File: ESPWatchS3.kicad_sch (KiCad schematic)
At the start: 128 parts

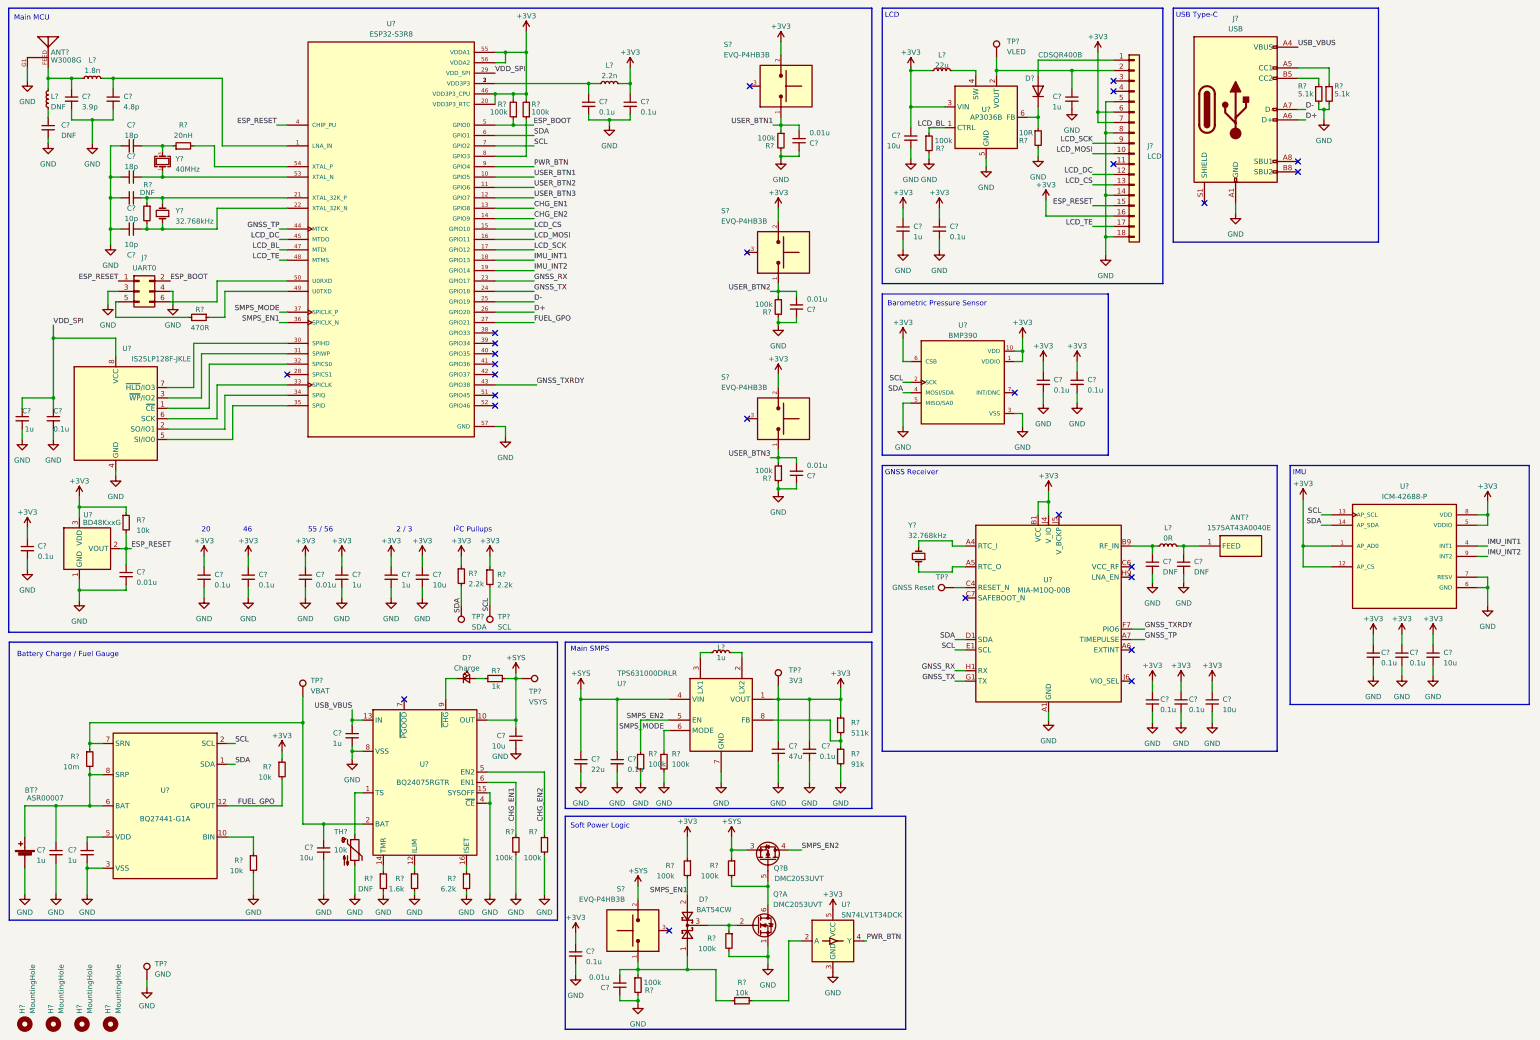
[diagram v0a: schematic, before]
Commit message: Re-annotated schematic
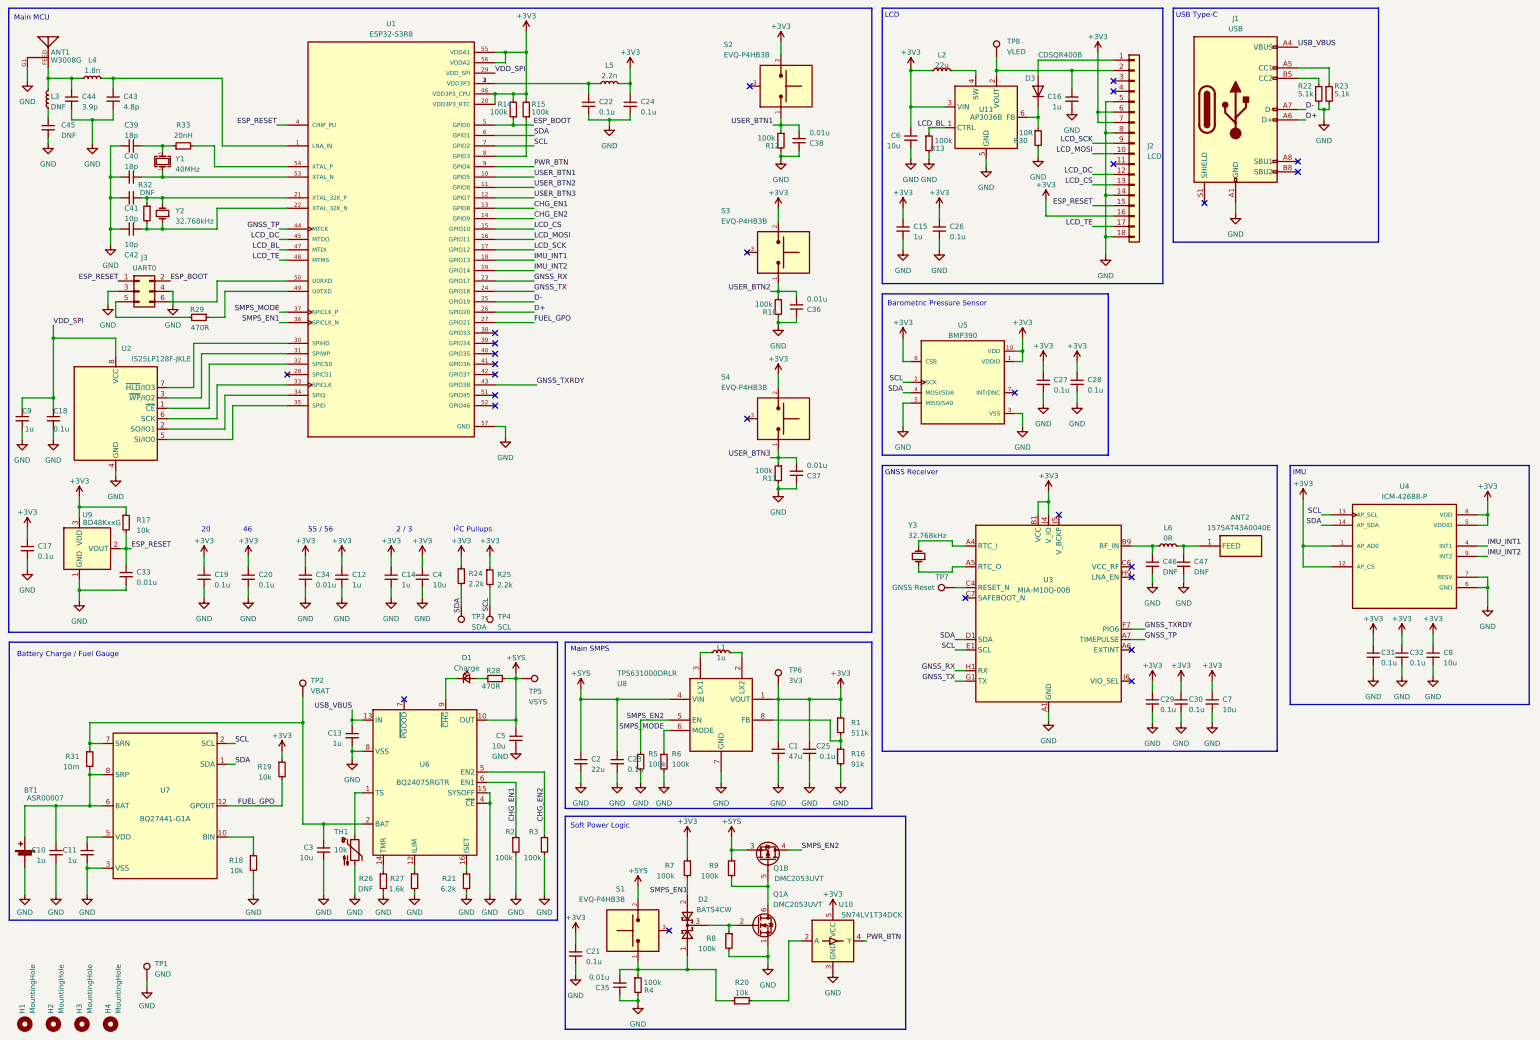
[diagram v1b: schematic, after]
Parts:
- R28: renamed from R?; value 1k -> 470R
- gave numbers to parts that had none: 126

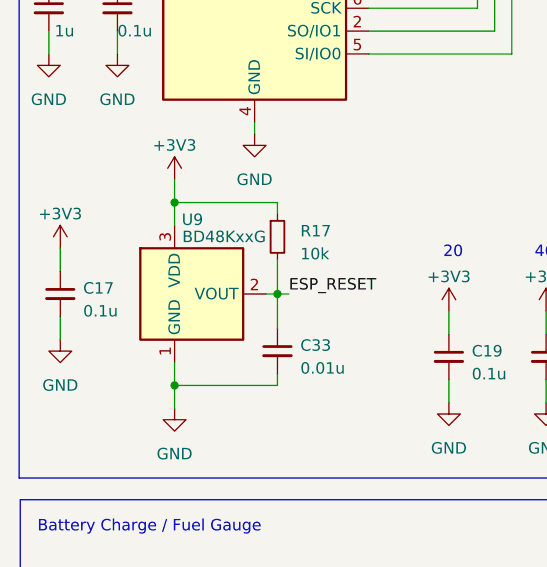
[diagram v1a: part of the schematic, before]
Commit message: Finished Footprint Assignment
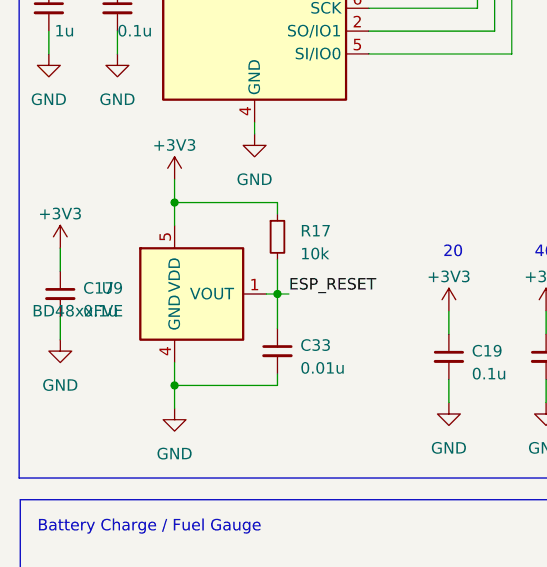
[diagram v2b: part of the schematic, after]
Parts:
- removed U9: BD48KxxG, Package_TO_SOT_SMD:SOT-23, symbol Power_Management:BD48KxxG
- added U9: BD48xxFVE, Package_TO_SOT_SMD:VSOF5, symbol Power_Management:BD48xxFVE
- J2: footprint (none) -> WatchParts:CS050Z18GA0
- L2: footprint (none) -> Inductor_SMD:L_1210_3225Metric
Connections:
- net +3V3: now also U9.5 (VDD)
- net EP: now also U9.2 (GND), U9.4 (GND)
- net ESP_RESET: now also U9.1 (VOUT)
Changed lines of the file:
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@@
       (effects (font (size 1.27 1.27)) (justify left))
     )
-    (property "Footprint" "" (at 288.925 46.99 0)
+    (property "Footprint" "WatchParts:CS050Z18GA0" (at 288.925 46.99 0)
       (effects (font (size 1.27 1.27)) hide)
     )
@@
       (effects (font (size 1.27 1.27)))
     )
-    (property "Footprint" "" (at 241.935 29.21 0)
+    (property "Footprint" "Inductor_SMD:L_1210_3225Metric" (at 241.935 29.21 0)
       (effects (font (size 1.27 1.27)) hide)
     )
@@
     )
   )
-  (symbol (lib_id "Power_Management:BD48KxxG") (at 31.115 146.05 0) (unit 1)
-    (in_bom yes) (on_board yes) (dnp no)
-    (property "Reference" "U9" (at 34.29 137.795 0)
-      (effects (font (size 1.27 1.27)) (justify right))
-    )
-    (property "Value" "BD48KxxG" (at 41.275 139.7 0)
-      (effects (font (size 1.27 1.27)) (justify right))
-    )
-    (property "Footprint" "Package_TO_SOT_SMD:SOT-23" (at 31.115 158.75 0)
-      (effects (font (size 1.27 1.27)) hide)
-    )
-    (property "Datasheet" "https://www.rohm.de/datasheet/BD4830FVE/bd48xxg-e" (at 31.115 161.29 0)
-      (effects (font (size 1.27 1.27)) hide)
-    )
-    (pin "1")
-    (pin "2")
-    (pin "3")
-    (instances
-      (project "ESPWatchS3"
-        (path "/bf5b2c41-bb33-4360-ba29-22d569e03292"
-          (reference "U9") (unit 1)
-        )
-      )
-    )
-  )
   (symbol (lib_id "Device:R_Small") (at 217.17 196.85 0) (unit 1)
     (in_bom yes) (on_board yes) (dnp no) (fields_autoplaced)
@@
         )
       )
+    )
+  )
+  (symbol (lib_id "Power_Management:BD48xxFVE") (at 31.115 146.05 0) (unit 1)
+    (in_bom yes) (on_board yes) (dnp no) (fields_autoplaced)
+    (property "Reference" "U9" (at 25.4 145.415 0)
+      (effects (font (size 1.27 1.27)) (justify right))
+    )
+    (property "Value" "BD48xxFVE" (at 25.4 147.955 0)
+      (effects (font (size 1.27 1.27)) (justify right))
+    )
+    (property "Footprint" "Package_TO_SOT_SMD:VSOF5" (at 31.115 158.75 0)
+      (effects (font (size 1.27 1.27)) hide)
+    )
+    (property "Datasheet" "https://www.rohm.de/datasheet/BD4830FVE/bd48xxg-e" (at 31.115 161.29 0)
+      (effects (font (size 1.27 1.27)) hide)
+    )
+    (pin "1")
+    (pin "2")
+    (pin "4")
+    (pin "5")
+    (instances
+      (project "ESPWatchS3"
+        (path "/bf5b2c41-bb33-4360-ba29-22d569e03292"
+          (reference "U9") (unit 1)
+        )
+      )
